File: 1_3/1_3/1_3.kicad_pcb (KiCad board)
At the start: 2 copper layers, 137.5 x 91.4 mm, 52 parts, among them SW1 SW_SPST, SW10 SW_SPST, SW11 SW_SPST, SW12 SW_SPST, SW13 SW_SPST, SW14 SW_SPST, SW15 SW_SPST, SW16 SW_SPST, SW17 SW_SPST, SW18 SW_SPST, SW19 SW_SPST, SW2 SW_SPST, SW20 SW_SPST, SW21 SW_SPST, SW3 SW_SPST, SW4 SW_SPST, SW5 SW_SPST, SW6 SW_SPST, SW7 SW_SPST, SW8 SW_SPST, SW9 SW_SPST, U1 XIAO_nRF52840

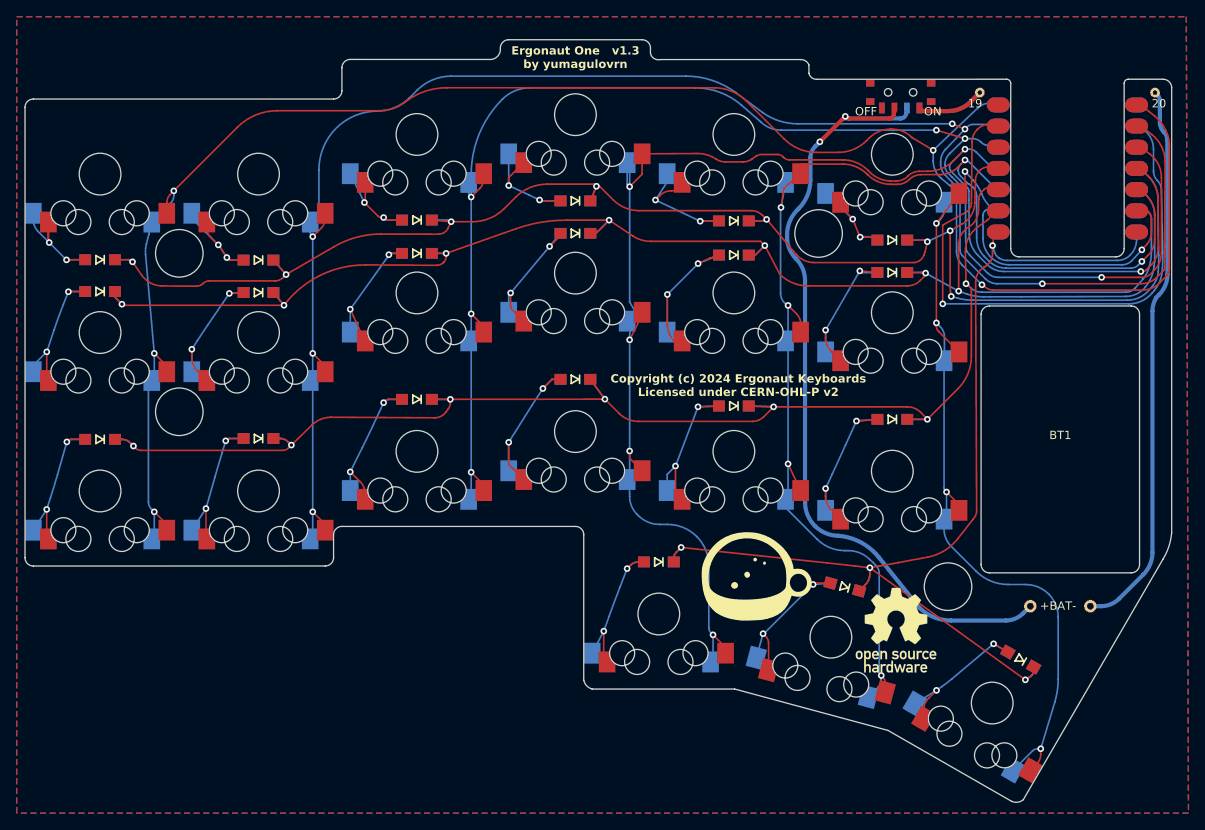
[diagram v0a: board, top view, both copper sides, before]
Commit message: 1_3 chk
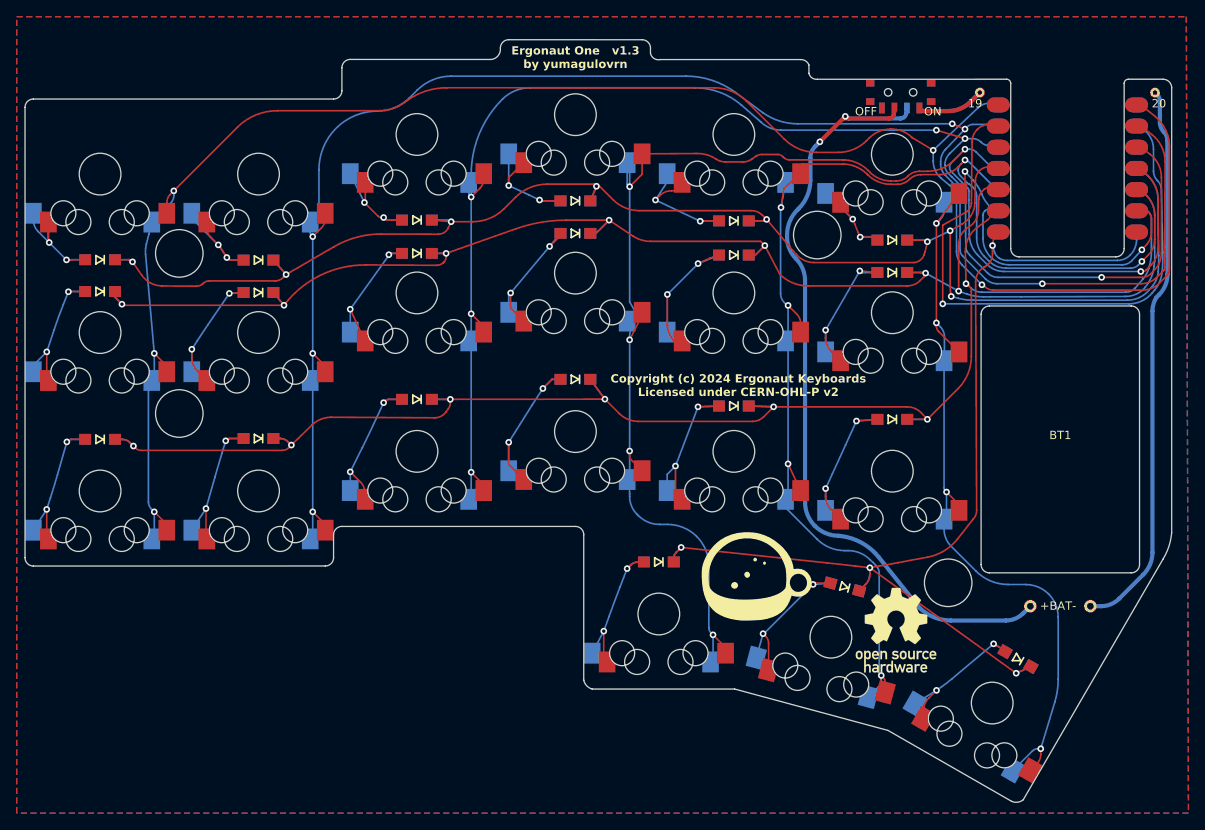
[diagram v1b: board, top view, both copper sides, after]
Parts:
- moved H4 0.46 mm to (186.2, 116.0)
- moved D21 0.33 mm to (194.6, 125.1)
- moved H3 0.25 mm to (170.5, 74.3)
- moved H2 0.21 mm to (94.0, 95.7)
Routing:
- net R3: track 128.7 -> 128.1 mm
